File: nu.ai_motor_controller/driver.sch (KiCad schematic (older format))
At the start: 8 parts, among them U5 MP6513, U6 MP6513, U7 MP6513, U8 MP6513

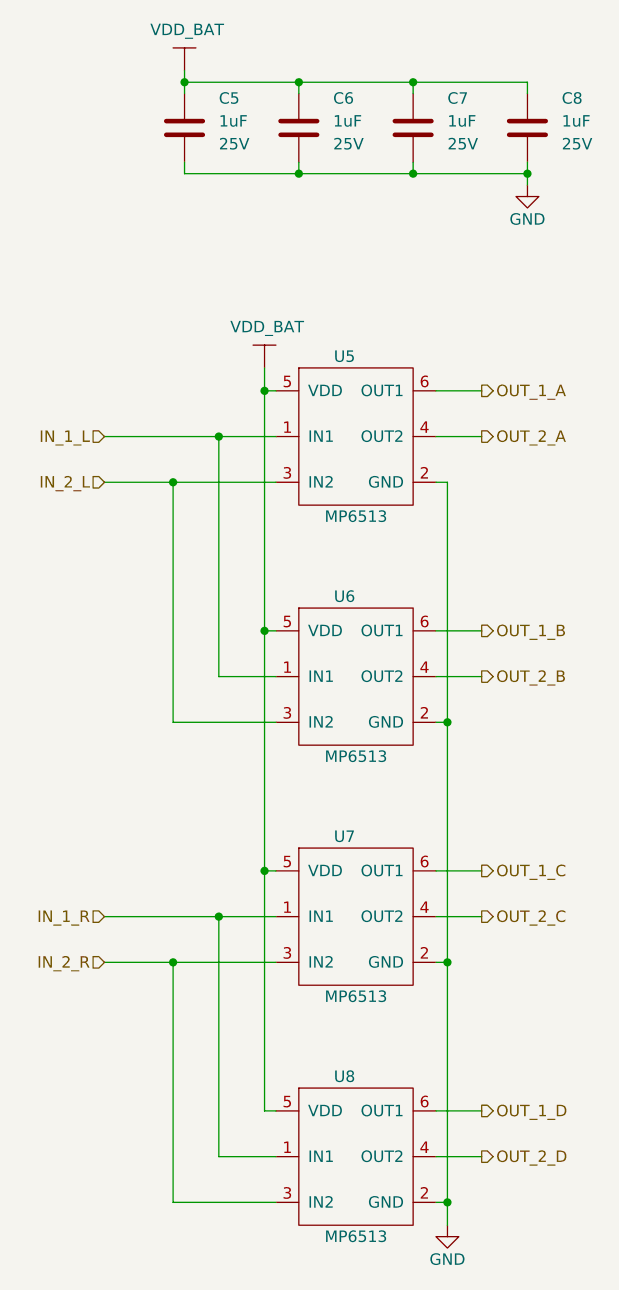
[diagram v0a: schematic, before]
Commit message: automated commit
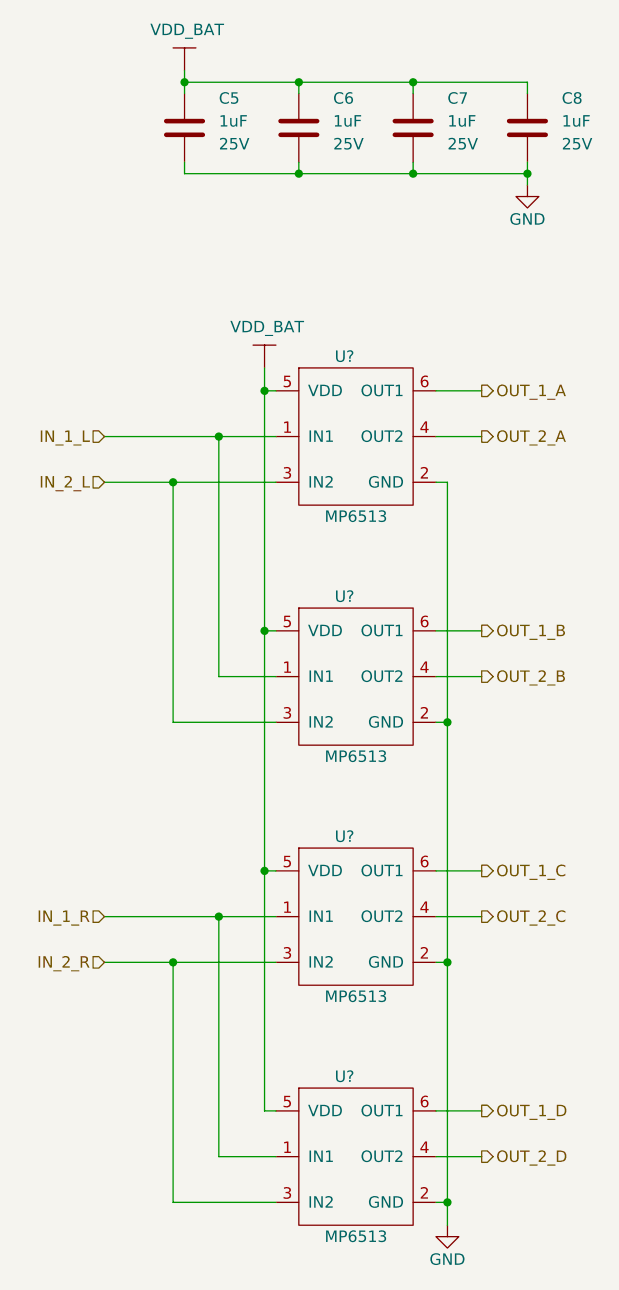
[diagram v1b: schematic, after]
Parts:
- removed U5, U6, U7, U8: MP6513, symbol custom:MP6513
- added U? (x4): MP6513, symbol custom:MP6513
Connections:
- net GND: now also U?.2 (GND), U?.2 (GND), U?.2 (GND), U?.2 (GND)
- net IN_1_L: now also U?.1 (IN1), U?.1 (IN1)
- net IN_1_R: now also U?.1 (IN1), U?.1 (IN1)
- net IN_2_L: now also U?.3 (IN2), U?.3 (IN2)
- net IN_2_R: now also U?.3 (IN2), U?.3 (IN2)
- net OUT_1_A: now also U?.6 (OUT1)
- net OUT_1_B: now also U?.6 (OUT1)
- net OUT_1_C: now also U?.6 (OUT1)
- net OUT_1_D: now also U?.6 (OUT1)
- net OUT_2_A: now also U?.4 (OUT2)
- net OUT_2_B: now also U?.4 (OUT2)
- net OUT_2_C: now also U?.4 (OUT2)
- net OUT_2_D: now also U?.4 (OUT2)
- net VDD_BAT: now also U?.5 (VDD), U?.5 (VDD), U?.5 (VDD), U?.5 (VDD)
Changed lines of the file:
@@
 Comment4 ""
 $EndDescr
-$Comp
-L custom:MP6513 U?
-U 1 1 5C101246
-P 4950 2650
-AR Path="/5C101246" Ref="U?"  Part="1"
-AR Path="/5C10107F/5C101246" Ref="U5"  Part="1"
-F 0 "U5" H 4900 3100 50  0000 C CNN
-F 1 "MP6513" H 4950 2400 50  0000 C CNN
-F 2 "" H 4950 2650 50  0001 C CNN
-F 3 "/home/dj/datasheet/MP6513.pdf" H 4950 2650 50  0001 C CNN
-	1    4950 2650
-	1    0    0    -1
-$EndComp
-$Comp
-L custom:MP6513 U?
-U 1 1 5C10124D
-P 4950 3700
-AR Path="/5C10124D" Ref="U?"  Part="1"
-AR Path="/5C10107F/5C10124D" Ref="U6"  Part="1"
-F 0 "U6" H 4900 4150 50  0000 C CNN
-F 1 "MP6513" H 4950 3450 50  0000 C CNN
-F 2 "" H 4950 3700 50  0001 C CNN
-F 3 "MP6513.pdf" H 4950 3700 50  0001 C CNN
-	1    4950 3700
-	1    0    0    -1
-$EndComp
-$Comp
-L custom:MP6513 U?
-U 1 1 5C101254
-P 4950 4750
-AR Path="/5C101254" Ref="U?"  Part="1"
-AR Path="/5C10107F/5C101254" Ref="U7"  Part="1"
-F 0 "U7" H 4900 5200 50  0000 C CNN
-F 1 "MP6513" H 4950 4500 50  0000 C CNN
-F 2 "" H 4950 4750 50  0001 C CNN
-F 3 "MP6513.pdf" H 4950 4750 50  0001 C CNN
-	1    4950 4750
-	1    0    0    -1
-$EndComp
-$Comp
-L custom:MP6513 U?
-U 1 1 5C10125B
-P 4950 5800
-AR Path="/5C10125B" Ref="U?"  Part="1"
-AR Path="/5C10107F/5C10125B" Ref="U8"  Part="1"
-F 0 "U8" H 4900 6250 50  0000 C CNN
-F 1 "MP6513" H 4950 5550 50  0000 C CNN
-F 2 "" H 4950 5800 50  0001 C CNN
-F 3 "MP6513.pdf" H 4950 5800 50  0001 C CNN
-	1    4950 5800
-	1    0    0    -1
-$EndComp
 Wire Wire Line
 	4600 5500 4550 5500
@@
 	1    0    0    -1
 $EndComp
+$Comp
+L custom:MP6513 U?
+U 1 1 5C565750
+P 4950 2650
+F 0 "U?" H 4900 3100 50  0000 C CNN
+F 1 "MP6513" H 4950 2400 50  0000 C CNN
+F 2 "" H 4950 2650 50  0001 C CNN
+F 3 "/home/dj/datasheets/MP6513.pdf" H 4950 2650 50  0001 C CNN
+	1    4950 2650
+	1    0    0    -1
+$EndComp
+$Comp
+L custom:MP6513 U?
+U 1 1 5C5657C3
+P 4950 3700
+F 0 "U?" H 4900 4150 50  0000 C CNN
+F 1 "MP6513" H 4950 3450 50  0000 C CNN
+F 2 "" H 4950 3700 50  0001 C CNN
+F 3 "/home/dj/datasheets/MP6513.pdf" H 4950 3700 50  0001 C CNN
+	1    4950 3700
+	1    0    0    -1
+$EndComp
+$Comp
+L custom:MP6513 U?
+U 1 1 5C565DC5
+P 4950 4750
+F 0 "U?" H 4900 5200 50  0000 C CNN
+F 1 "MP6513" H 4950 4500 50  0000 C CNN
+F 2 "" H 4950 4750 50  0001 C CNN
+F 3 "/home/dj/datasheets/MP6513.pdf" H 4950 4750 50  0001 C CNN
+	1    4950 4750
+	1    0    0    -1
+$EndComp
+$Comp
+L custom:MP6513 U?
+U 1 1 5C565E47
+P 4950 5800
+F 0 "U?" H 4900 6250 50  0000 C CNN
+F 1 "MP6513" H 4950 5550 50  0000 C CNN
+F 2 "" H 4950 5800 50  0001 C CNN
+F 3 "/home/dj/datasheets/MP6513.pdf" H 4950 5800 50  0001 C CNN
+	1    4950 5800
+	1    0    0    -1
+$EndComp

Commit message: automated commit
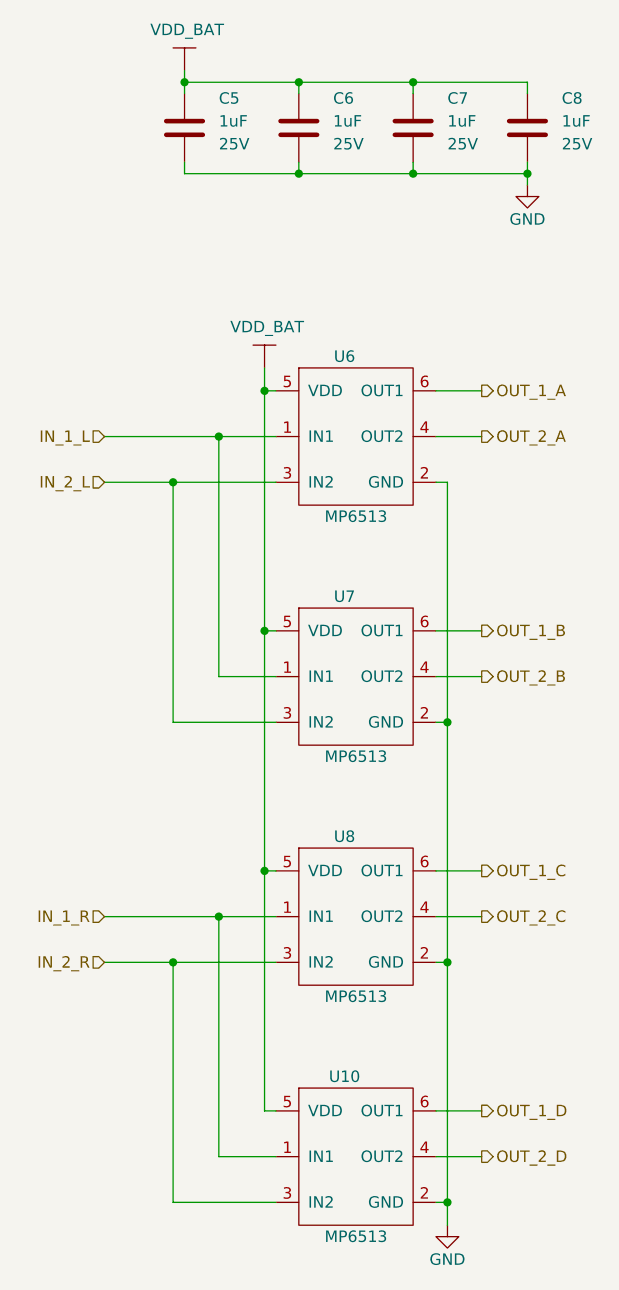
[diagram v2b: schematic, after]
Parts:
- gave numbers to parts that had none: 4
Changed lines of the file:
@@
 $EndComp
 $Comp
-L custom:MP6513 U?
+L custom:MP6513 U6
 U 1 1 5C565750
 P 4950 2650
-F 0 "U?" H 4900 3100 50  0000 C CNN
+F 0 "U6" H 4900 3100 50  0000 C CNN
 F 1 "MP6513" H 4950 2400 50  0000 C CNN
 F 2 "" H 4950 2650 50  0001 C CNN
@@
 $EndComp
 $Comp
-L custom:MP6513 U?
+L custom:MP6513 U7
 U 1 1 5C5657C3
 P 4950 3700
-F 0 "U?" H 4900 4150 50  0000 C CNN
+F 0 "U7" H 4900 4150 50  0000 C CNN
 F 1 "MP6513" H 4950 3450 50  0000 C CNN
 F 2 "" H 4950 3700 50  0001 C CNN
@@
 $EndComp
 $Comp
-L custom:MP6513 U?
+L custom:MP6513 U8
 U 1 1 5C565DC5
 P 4950 4750
-F 0 "U?" H 4900 5200 50  0000 C CNN
+F 0 "U8" H 4900 5200 50  0000 C CNN
 F 1 "MP6513" H 4950 4500 50  0000 C CNN
 F 2 "" H 4950 4750 50  0001 C CNN
@@
 $EndComp
 $Comp
-L custom:MP6513 U?
+L custom:MP6513 U10
 U 1 1 5C565E47
 P 4950 5800
-F 0 "U?" H 4900 6250 50  0000 C CNN
+F 0 "U10" H 4900 6250 50  0000 C CNN
 F 1 "MP6513" H 4950 5550 50  0000 C CNN
 F 2 "" H 4950 5800 50  0001 C CNN
